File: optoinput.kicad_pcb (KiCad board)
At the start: 2 copper layers, 76.2 x 50.8 mm, 32 parts, among them P1 CONN_01X08, P2 CONN_01X08, P3 CONN_01X03, P6 CONN_01X02, U1 4N25, U2 4N25, U3 4N25, U4 4N25, U5 4N25, U6 4N25, U7 4N25, U8 4N25

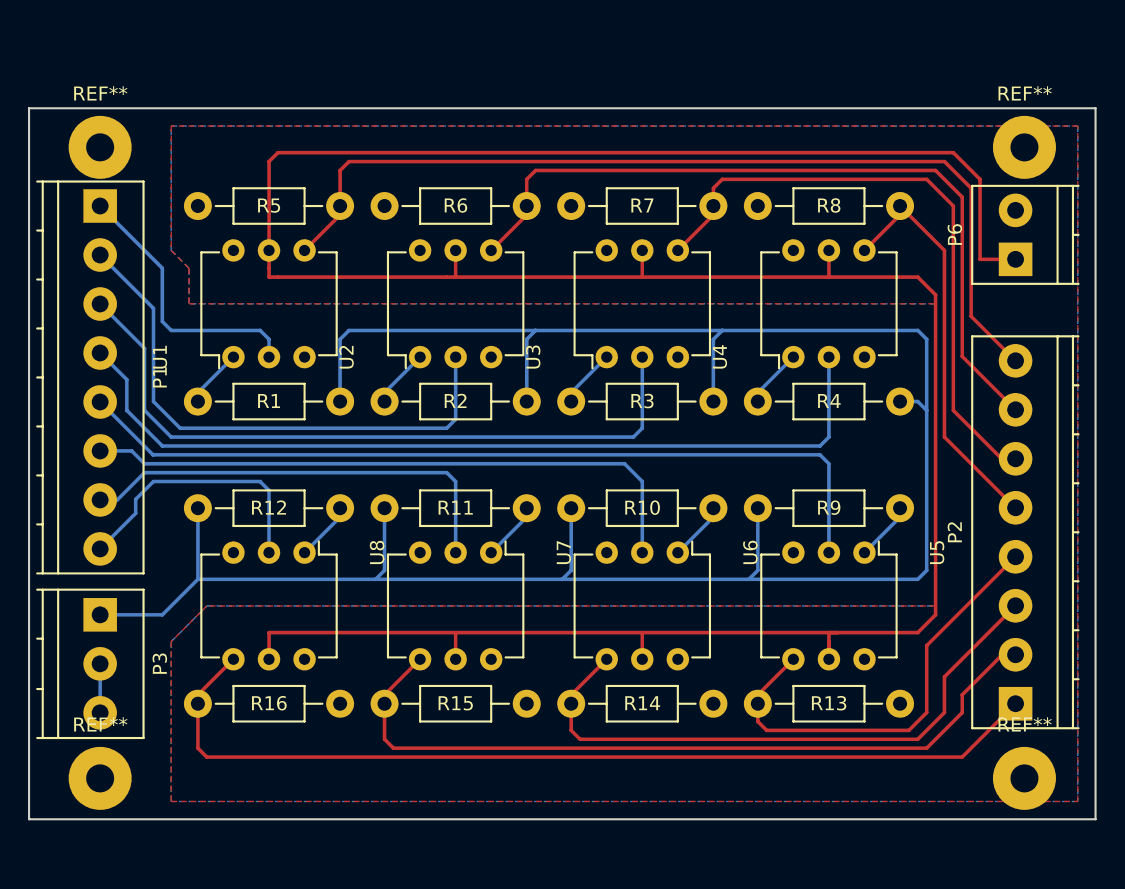
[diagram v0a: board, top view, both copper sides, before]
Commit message: single layer mod
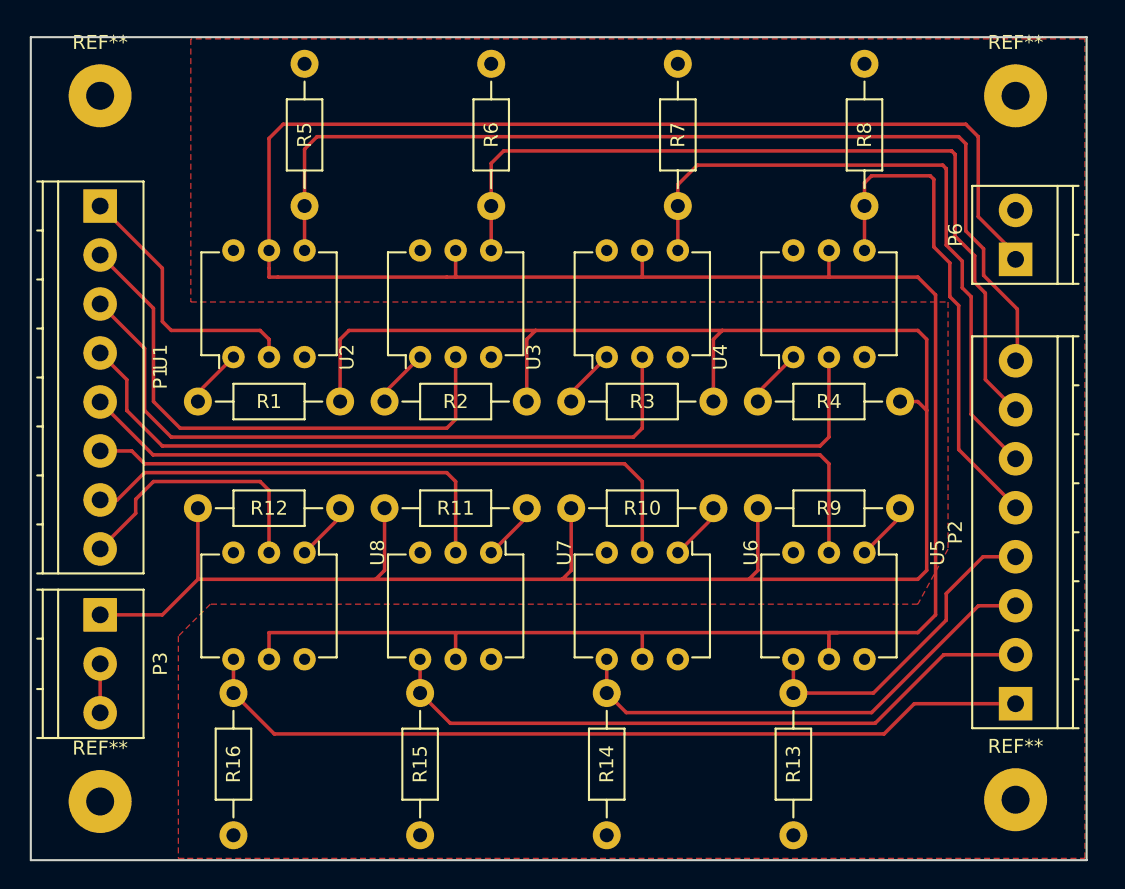
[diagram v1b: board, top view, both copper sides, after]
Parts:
- REF** (x4): value SolderWirePad_single_2mmDrill -> 2mm
- moved REF** 3.74 mm to (102.2, 48.6)
- moved REF** 3.68 mm to (36.8, 48.6)
- moved R13 2.65 mm to (86.4, 91.3), turned to 270 degrees
- moved R14 2.65 mm to (73.0, 91.3), turned to 270 degrees
- moved R15 2.65 mm to (59.7, 91.3), turned to 270 degrees
- moved R16 2.65 mm to (46.4, 91.3), turned to 270 degrees
- moved R6 2.54 mm to (64.8, 56.5), turned to 90 degrees
- moved R8 2.54 mm to (91.4, 56.5), turned to 90 degrees
- moved R5 2.54 mm to (51.4, 56.5), turned to 90 degrees
- moved R7 2.54 mm to (78.1, 56.5), turned to 90 degrees
- moved REF** 1.65 mm to (102.2, 98.9)
- moved REF** 1.65 mm to (36.8, 99.1)
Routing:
- net /Y5: track 32.1 -> 23.5 mm
- net /Y6: track 43.6 -> 35.4 mm
- net /Y8: track 67.7 -> 60.4 mm
- net /Y7: track 55.6 -> 48.8 mm
- net /Y4: track 29.2 -> 36.0 mm
- net /Y1: track 66.5 -> 72.1 mm
- net /Y2: track 55.1 -> 59.9 mm
- net /Y3: track 44.2 -> 48.3 mm
- net VCC: track 202.8 -> 205.6 mm
- removed copper zone on B.Cu, net GND
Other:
- board size 76.2 x 50.8 mm -> 75.4 x 58.8 mm
